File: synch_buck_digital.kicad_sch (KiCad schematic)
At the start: 49 parts, among them U1 BSC066N06NSATMA1, U2 BSC066N06NSATMA1, U3 INA241A3IDDFR

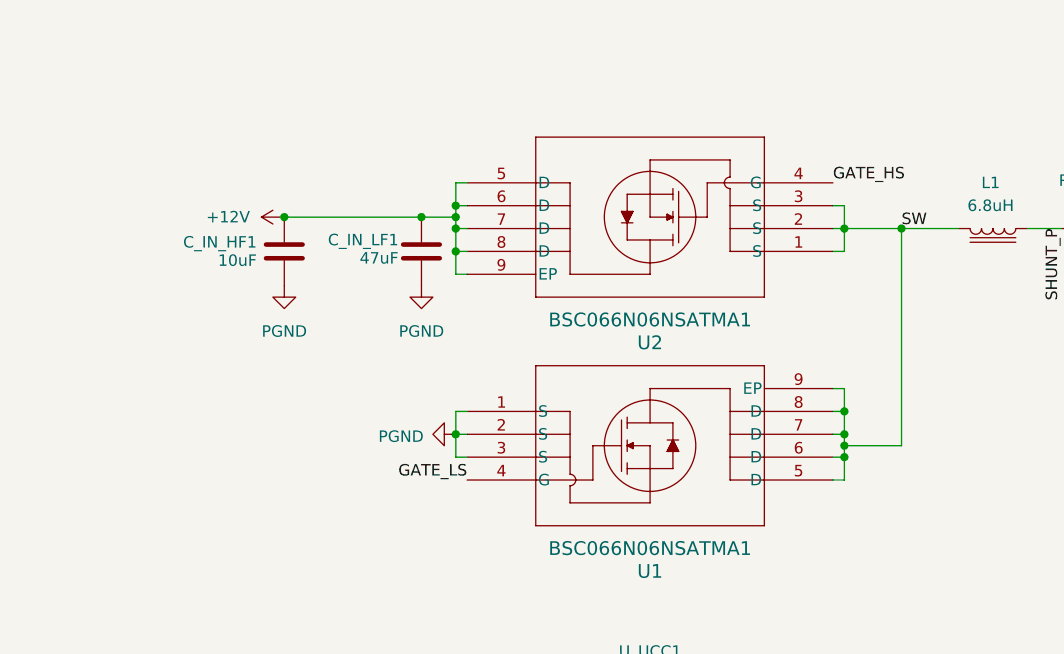
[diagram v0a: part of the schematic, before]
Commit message: V1 finished. Final touchups to schematic planned
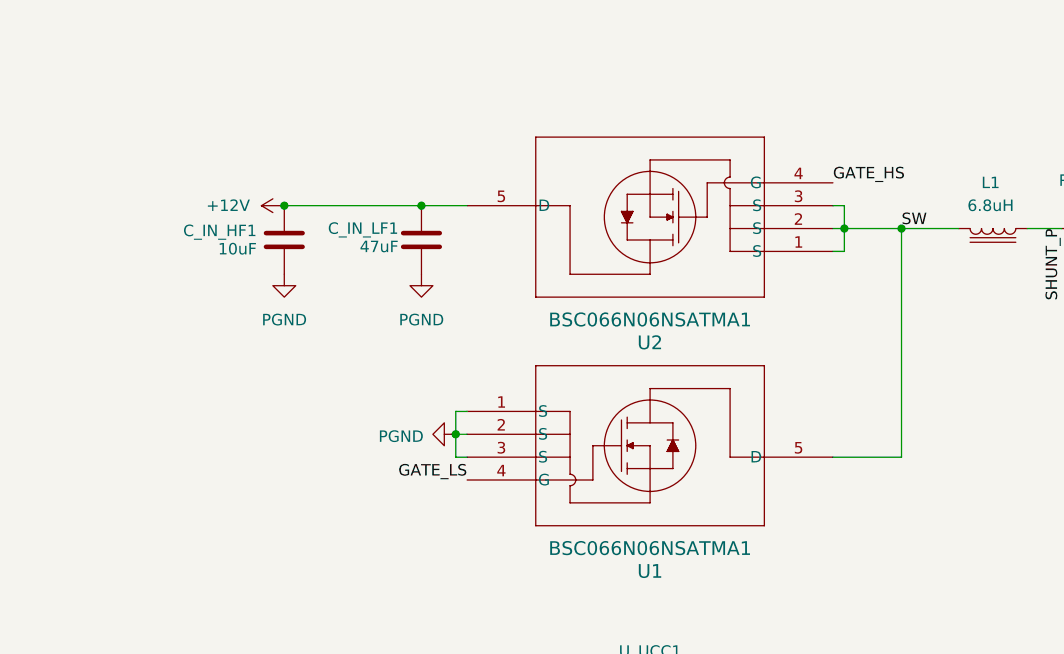
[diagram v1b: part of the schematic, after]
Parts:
- U1, U2: footprint PG-TDSON-8_INF -> Package_SON:Infineon_PG-TDSON-8_6.15x5.15mm
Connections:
- net +12V: no longer U2.6 (D), U2.7 (D), U2.8 (D), U2.9 (EP)
- net SW: no longer U1.6 (D), U1.7 (D), U1.8 (D), U1.9 (EP)
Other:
- moved on the sheet: C_IN_HF1, C_IN_LF1
